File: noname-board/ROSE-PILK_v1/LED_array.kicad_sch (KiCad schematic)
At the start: 1 part, among them U6 CD4514BM

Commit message: Board Design WIP
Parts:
- U6: footprint CD4514BM:DW24 -> CD4514BM:SOIC127P1030X265-24N
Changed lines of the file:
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@@
       (effects (font (size 1.27 1.27)))
     )
-    (property "Footprint" "CD4514BM:DW24" (at 134.62 85.09 0)
+    (property "Footprint" "CD4514BM:SOIC127P1030X265-24N" (at 134.62 85.09 0)
       (effects (font (size 1.27 1.27)) (justify bottom) hide)
     )

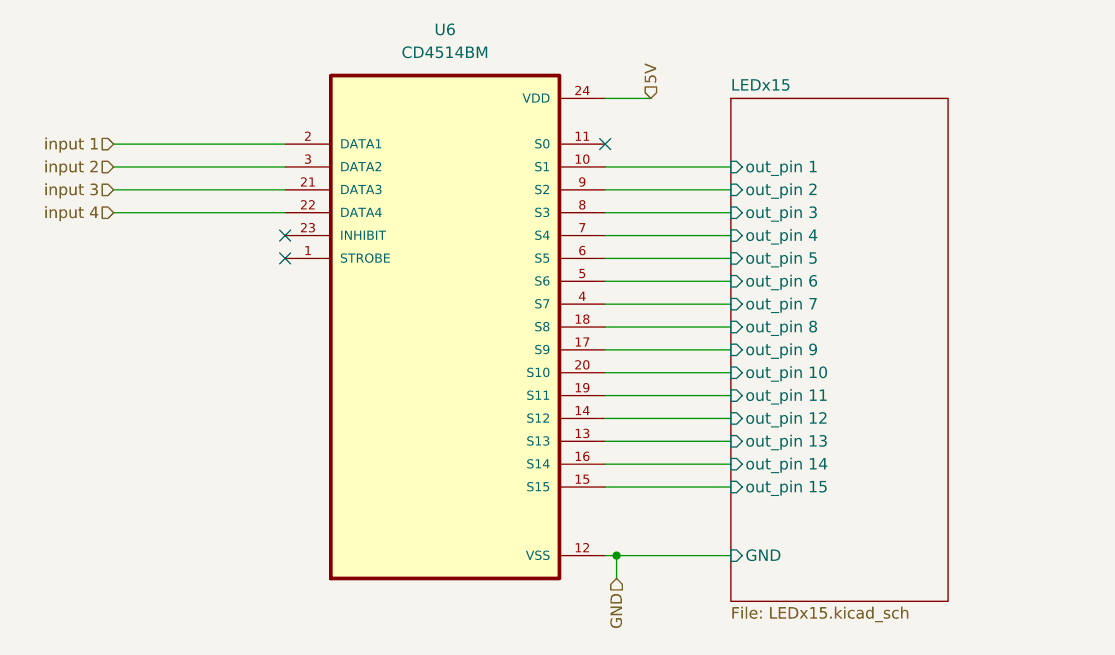
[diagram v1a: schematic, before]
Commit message: LED Array
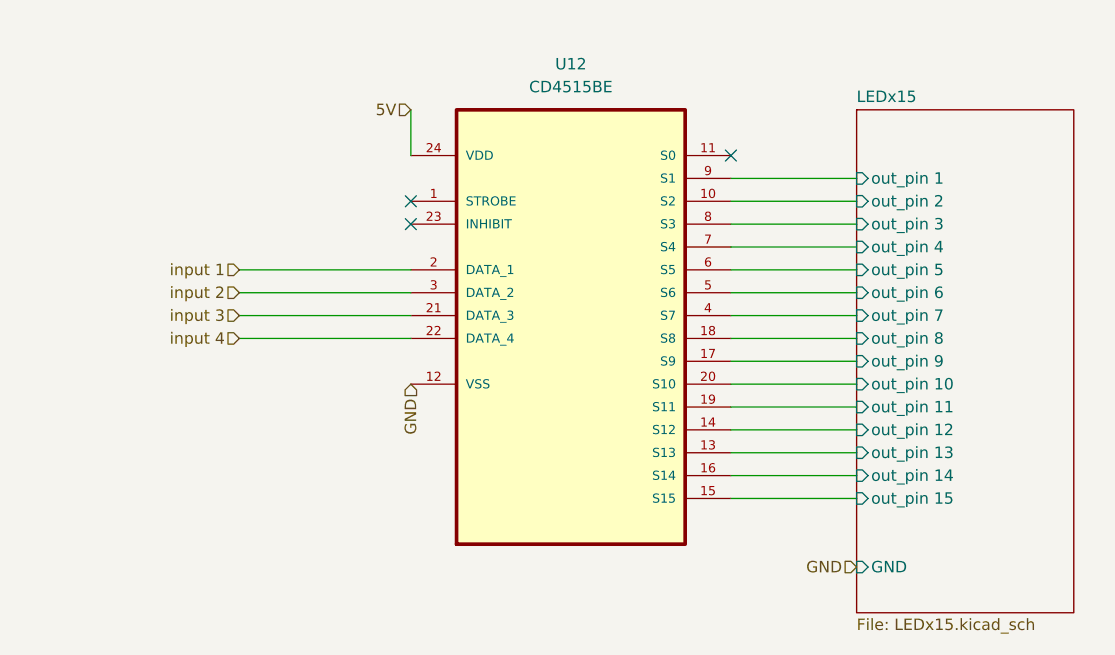
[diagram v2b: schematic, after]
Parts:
- removed U6: CD4514BM, CD4514BM:SOIC127P1030X265-24N, symbol CD4514BM:CD4514BM
- added U12: CD4515BE, CD4515BE:DIP254P1080X508-24, symbol CD4515BE:CD4515BE
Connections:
- net 5V: now also U12.24 (VDD)
- net GND: now also U12.12 (VSS)
- net LEDx15/out_pin 1: now also U12.9 (S1)
- net LEDx15/out_pin 10: now also U12.20 (S10)
- net LEDx15/out_pin 11: now also U12.19 (S11)
- net LEDx15/out_pin 12: now also U12.14 (S12)
- net LEDx15/out_pin 13: now also U12.13 (S13)
- net LEDx15/out_pin 14: now also U12.16 (S14)
- net LEDx15/out_pin 15: now also U12.15 (S15)
- net LEDx15/out_pin 2: now also U12.10 (S2)
- net LEDx15/out_pin 3: now also U12.8 (S3)
- net LEDx15/out_pin 4: now also U12.7 (S4)
- net LEDx15/out_pin 5: now also U12.6 (S5)
- net LEDx15/out_pin 6: now also U12.5 (S6)
- net LEDx15/out_pin 7: now also U12.4 (S7)
- net LEDx15/out_pin 8: now also U12.18 (S8)
- net LEDx15/out_pin 9: now also U12.17 (S9)
- net input 1: now also U12.2 (DATA_1)
- net input 2: now also U12.3 (DATA_2)
- net input 3: now also U12.21 (DATA_3)
- net input 4: now also U12.22 (DATA_4)
